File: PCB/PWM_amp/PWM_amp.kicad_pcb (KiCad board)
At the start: 2 copper layers, 84 x 84 mm, 47 parts, among them J1 Conn_01x06_Pin, J10 XT30UPB-M, J2 Conn_01x06_Pin, J3 Conn_01x02_Pin, J4 Conn_01x02_Pin, J49 XT60PW-M, J5 XT30UPB-M, Q1 FDD8447L, Q2 FDD8447L, U1 VNH5019A-E, U2 VNH5019A-E, U3 NC7SVU04P5X, U4 NC7SVU04P5X

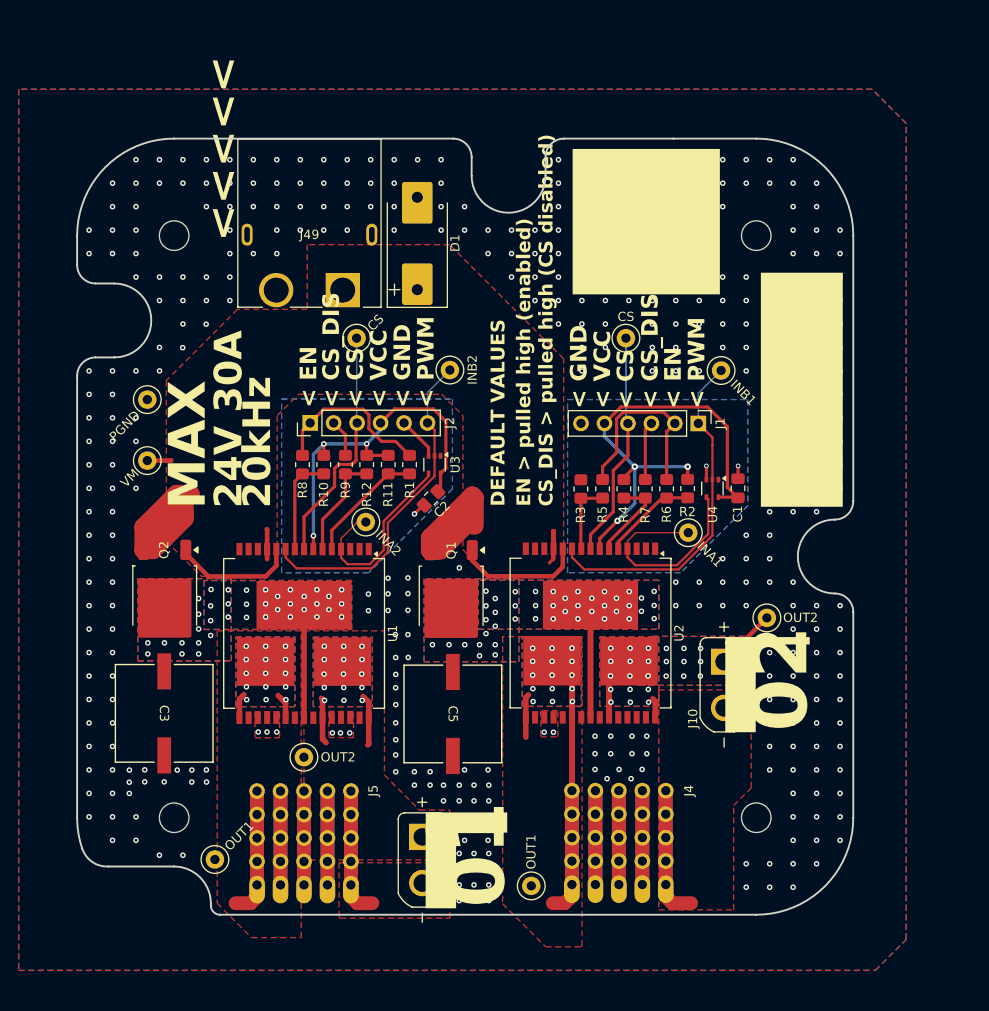
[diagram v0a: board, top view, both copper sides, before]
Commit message: 3d models and PCB
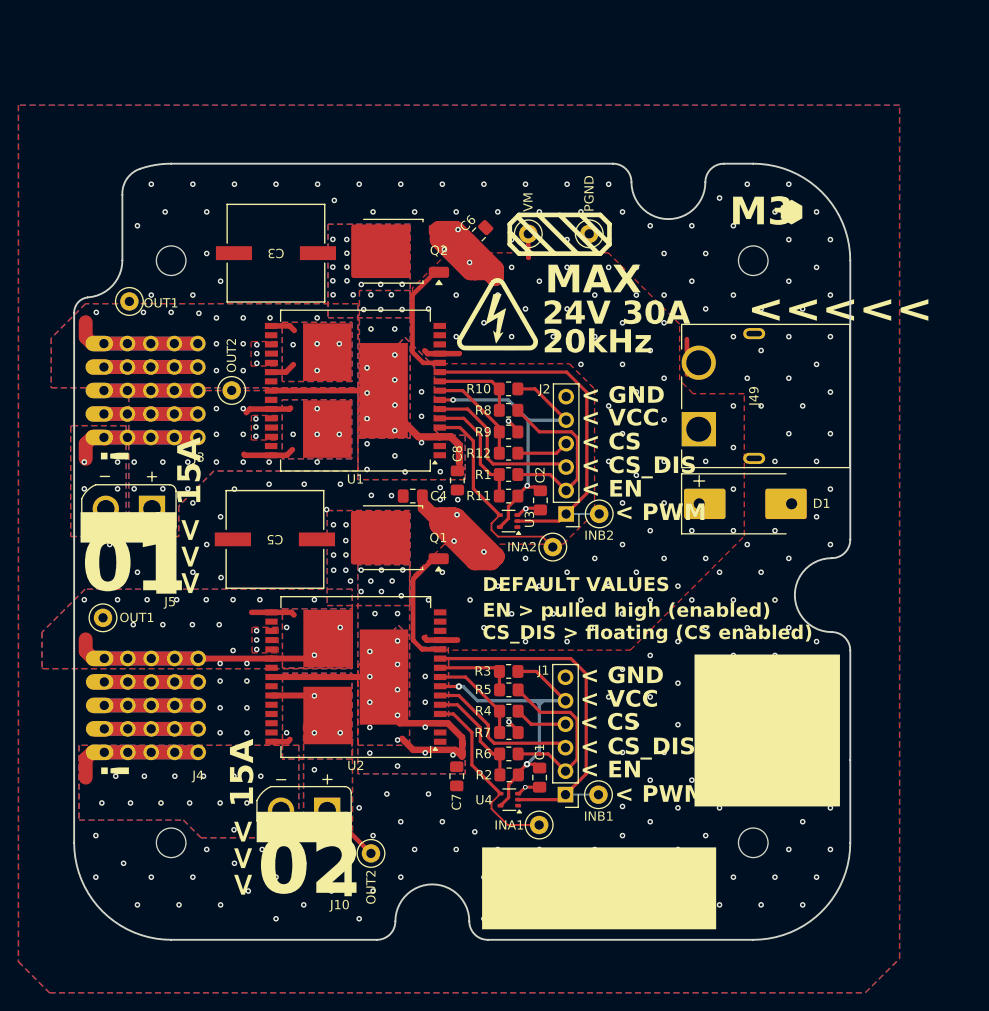
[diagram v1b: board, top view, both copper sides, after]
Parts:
- removed CS (x2): CS, TestPoint:TestPoint_Loop_D1.80mm_Drill1.0mm_Beaded
- added C4: 1uF, Capacitor_SMD:C_0805_2012Metric_Pad1.18x1.45mm_HandSolder, F.Cu at (226.8, 116.4)
- added C6: 1uF, Capacitor_SMD:C_0805_2012Metric_Pad1.18x1.45mm_HandSolder, F.Cu at (233.9, 88.1)
- added C7: 0.1uF, Capacitor_SMD:C_0805_2012Metric_Pad1.18x1.45mm_HandSolder, F.Cu at (231.5, 146.7)
- added C8: 0.1uF, Capacitor_SMD:C_0805_2012Metric_Pad1.18x1.45mm_HandSolder, F.Cu at (231.6, 114.7)
- added G***: LOGO, LOGO, F.Cu at (266.9, 104.3)
- added G***: LOGO, LOGO, F.Cu at (235.9, 96.8)
- added G***: LOGO, LOGO, F.Cu at (267.7, 85.7)
- added G***: LOGO, LOGO, B.Cu at (267.7, 85.7)
- moved H1 65.7 mm to (263.6, 153.9), turned to -90 degrees
- moved H2 63.4 mm to (200.6, 153.9), turned to -90 degrees
- moved H8 62.7 mm to (263.6, 90.9), turned to -90 degrees
- moved OUT1 61.1 mm to (196.1, 95.4), turned to -90 degrees
- moved H3 60.3 mm to (200.6, 90.9), turned to -90 degrees
- moved OUT1 54.7 mm to (193.2, 129.6), turned to -90 degrees
- moved C3 51.3 mm to (212.0, 90.1), turned to 180 degrees
- moved J49 51.2 mm to (263.7, 105.6), turned to 90 degrees
- moved PGND 51.1 mm to (245.9, 88.0), turned to -90 degrees
- moved OUT2 49.9 mm to (222.2, 155.1), turned to -90 degrees
- moved J5 49.5 mm to (196.1, 117.8), turned to 180 degrees
- moved J3 48.9 mm to (203.5, 99.9), turned to 180 degrees
- moved VM 48.0 mm to (239.3, 88.0), turned to -90 degrees
- moved INB1 47.8 mm to (246.9, 148.7), turned to -90 degrees
- moved J10 47.5 mm to (215.0, 150.5), turned to 180 degrees
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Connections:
- J2 pad 1: Net-(J2-Pin_1) -> INB2
- J2 pad 4: +3V_1 -> Net-(J2-Pin_4)
- J2 pad 5: GND1 -> +3V_1
- J2 pad 6: INB2 -> GND1
- R1 pad 1: Net-(J2-Pin_1) -> Net-(J2-Pin_2)
- R12 pad 1: +3V_1 -> Net-(J2-Pin_4)
- R12 pad 2: Net-(U1-CS_DIS) -> Net-(U1-CS)
- R4 pad 1: +3V_1 -> Net-(J1-Pin_4)
- R4 pad 2: Net-(U2-CS_DIS) -> Net-(U2-CS)
- R7 pad 1: Net-(J1-Pin_3) -> GND1
- R7 pad 2: Net-(U2-CS_DIS) -> Net-(U2-CS)
- R8 pad 1: Net-(J2-Pin_1) -> Net-(J2-Pin_2)
- R9 pad 1: Net-(J2-Pin_2) -> GND1
- R9 pad 2: Net-(U1-CS_DIS) -> Net-(U1-CS)
- U1 pad 6: Net-(U1-CS_DIS) -> Net-(J2-Pin_3)
- U1 pad 8: Net-(J2-Pin_3) -> Net-(U1-CS)
- U2 pad 6: Net-(U2-CS_DIS) -> Net-(J1-Pin_3)
- U2 pad 8: Net-(J1-Pin_4) -> Net-(U2-CS)
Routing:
- net Net-(Q1-D): track 12.2 -> 32.5 mm, vias 43 -> 34
- net Net-(J1-Pin_4): track 24.6 -> 5.72 mm
- net Net-(J2-Pin_1): track 18.2 -> 0.00 mm
- net +3V_1: track 91.4 -> 75.3 mm, vias 6 -> 4
- net Net-(Q2-D): track 12.2 -> 28.1 mm, vias 38 -> 34
- net Net-(J2-Pin_2): track 4.04 -> 19.9 mm
- net Net-(U1-CS_DIS): track 11.5 -> 0.00 mm
- net Net-(U2-CS): track 0.00 -> 11.3 mm
- net Net-(U1-CS): track 0.00 -> 11.0 mm
- net Net-(J1-Pin_3): track 6.35 -> 16.7 mm
- net Net-(U2-CS_DIS): track 9.43 -> 0.00 mm
- net Net-(J2-Pin_3): track 26.1 -> 18.1 mm
- net VM1: track 63.0 -> 57.2 mm, vias 0 -> 67
- net Net-(J2-Pin_4): track 0.00 -> 5.74 mm
- net INB2: track 36.8 -> 40.2 mm
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- added copper zone on In1.Cu, net GND1
- added copper zone on B.Cu, net Net-(J3-Pin_2)
- added copper zone on B.Cu, net Net-(J4-Pin_2)
- added copper zone on In2.Cu, net Net-(Q1-D)
- added copper zone on In2.Cu, net Net-(Q2-D)
- added copper zone on In1.Cu, net PGND1
- added copper zone on In2.Cu, net VM1
- removed copper zone on B.Cu, net GND1
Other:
- outline, holes or cut-outs redrawn
- copper layers 2 -> 4
- board text added: "!"
- board text added: "24V"
- board text added: "4/Mar 2026 Iter. 1.1.0"
- board text added: "<<< 15A"
- board text added: "EN > pulled high (enabled) CS_DIS > floating (CS enabled)"
- board text added: "J3"
- board text added: "M3"
- board text removed: "1/Mar 2026 Ver. 1.0"
- board text removed: "EN > pulled high (enabled) CS_DIS > pulled high (CS disabled)"
